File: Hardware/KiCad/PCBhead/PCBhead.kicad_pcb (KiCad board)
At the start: 2 copper layers, 32 x 32 mm, 10 parts, among them IC2 OPT3002DNPT, J1 LEDazul, J2 LEDambar, J4 Vin

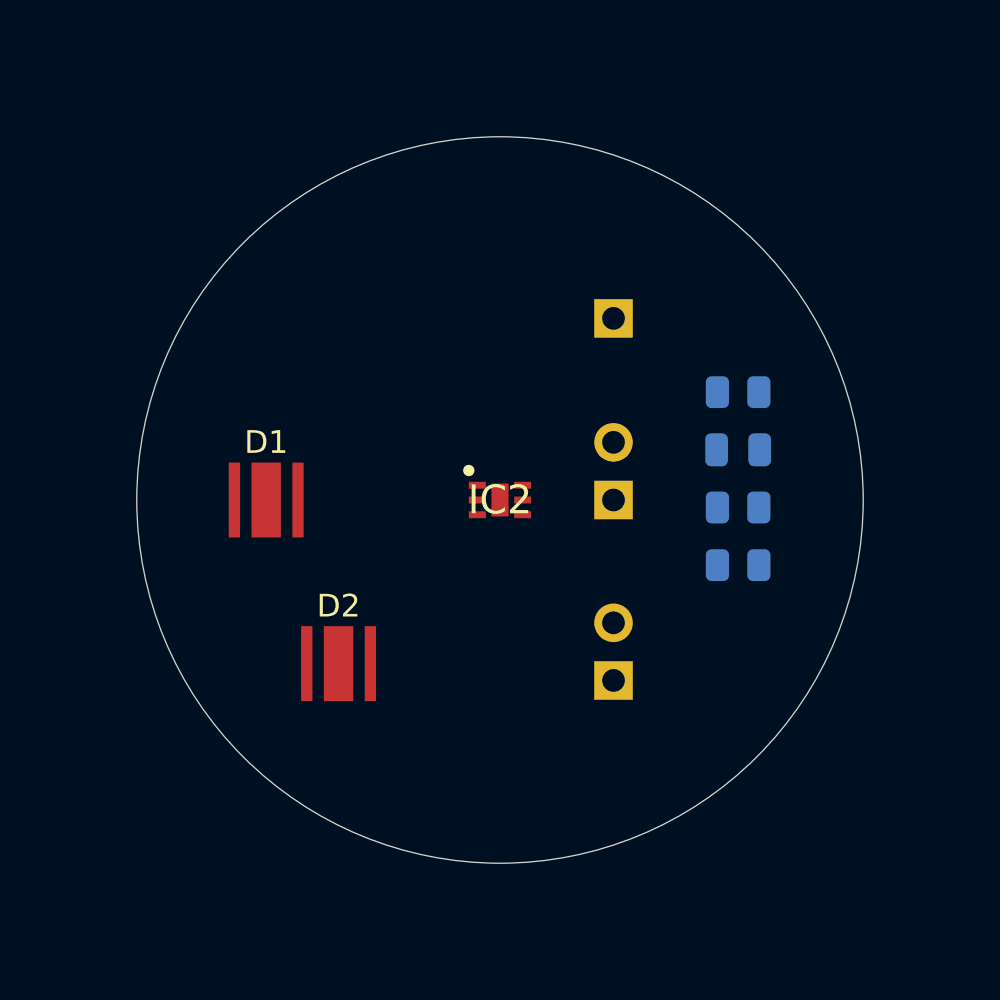
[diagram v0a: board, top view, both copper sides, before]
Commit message: head update
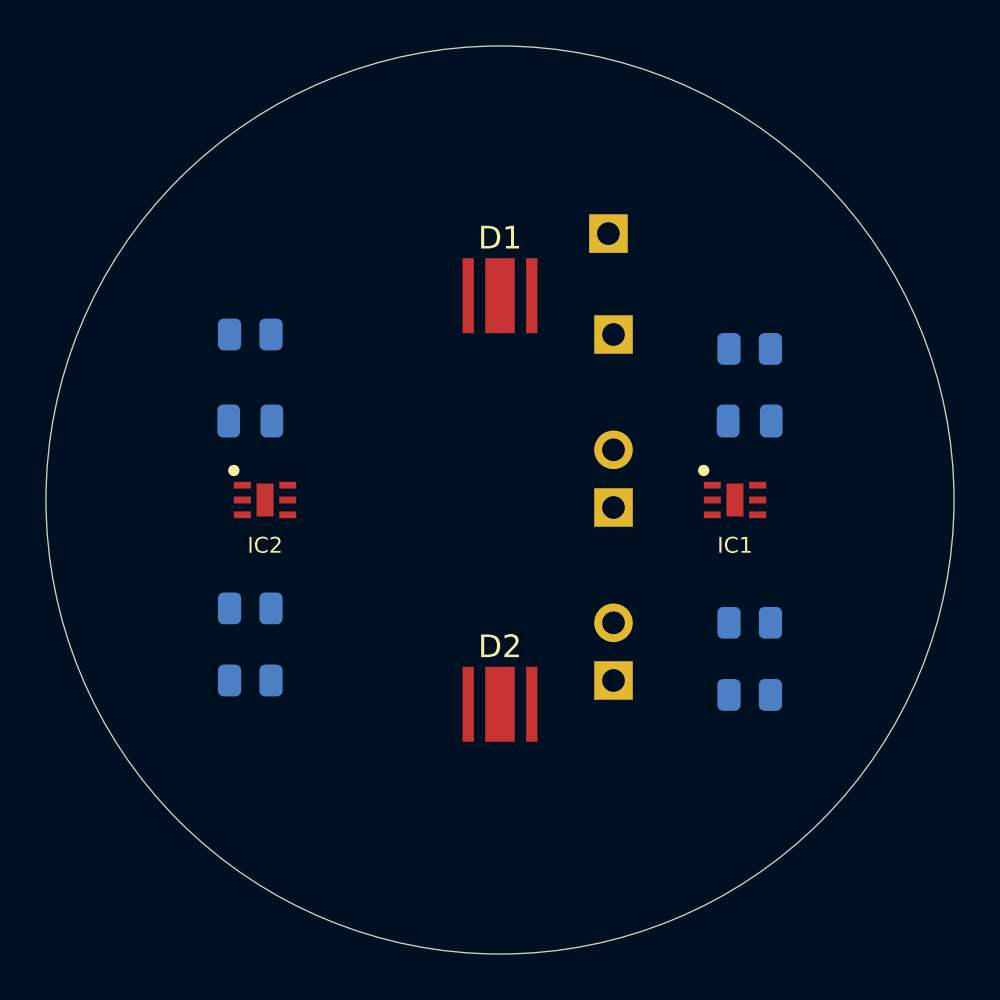
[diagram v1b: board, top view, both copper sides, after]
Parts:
- added C1: C_Small, Capacitor_SMD:C_0805_2012Metric, B.Cu at (89.0, 96.5)
- added IC1: OPT3002DNPT, OPT3002DNPT:SON65P200X200X65-7N-D, F.Cu at (110.3, 100.0)
- added J3: Vin, Connector_PinSocket_2.54mm:PinSocket_1x01_P2.54mm_Horizontal, B.Cu at (104.8, 88.3)
- added R1: 10k, Resistor_SMD:R_0805_2012Metric, B.Cu at (89.0, 108.0)
- added R2: 10k, Resistor_SMD:R_0805_2012Metric, B.Cu at (89.0, 92.7)
- added R3: 10k, Resistor_SMD:R_0805_2012Metric, B.Cu at (89.0, 104.8)
- moved D1 13.7 mm to (100.0, 91.0)
- moved IC2 10.3 mm to (89.7, 100.0)
- moved R6 8.27 mm to (111.0, 108.6)
- moved D2 7.33 mm to (100.0, 109.0)
- moved R5 2.59 mm to (111.0, 105.4)
- moved R4 1.97 mm to (111.0, 93.3)
- moved C2 1.37 mm to (111.0, 96.5)
- moved J4 0.71 mm to (105.0, 92.7)
- moved J1 0.33 mm to (105.0, 100.3)
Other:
- board size 32 x 32 mm -> 40 x 40 mm
